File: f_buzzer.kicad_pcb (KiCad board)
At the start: 2 copper layers, 71.5 x 44 mm, 0 parts

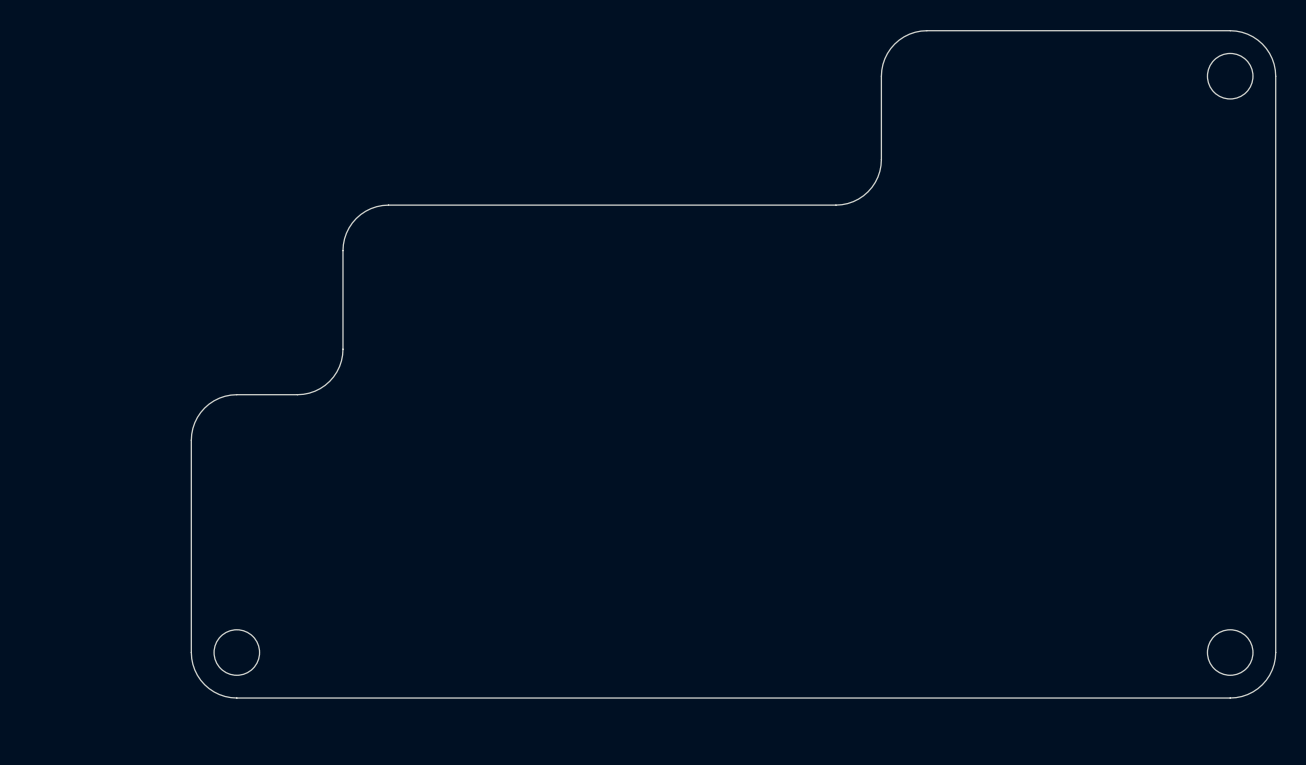
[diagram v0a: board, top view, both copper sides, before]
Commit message: Rev1
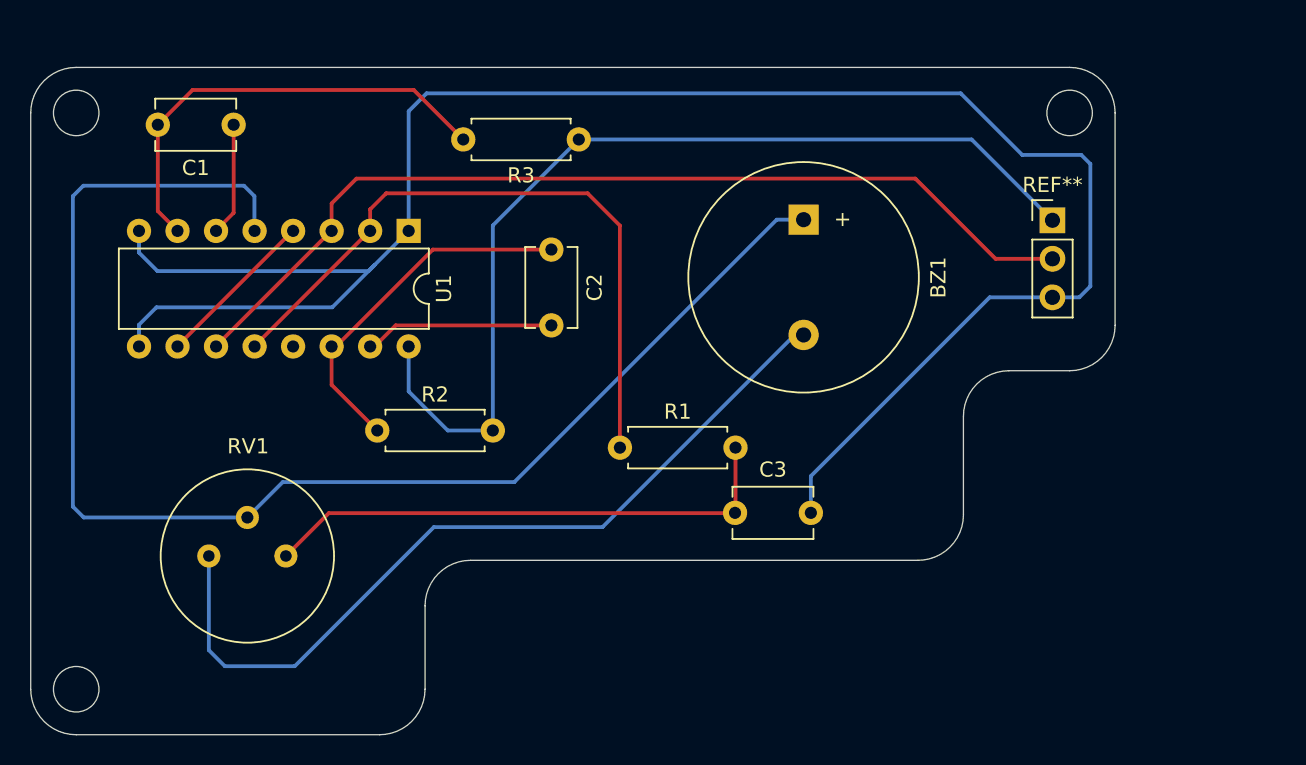
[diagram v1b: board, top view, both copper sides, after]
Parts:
- added BZ1: Buzzer, Buzzer_Beeper:Buzzer_15x7.5RM7.6, F.Cu at (165.2, 86.2)
- added C1: C, Capacitor_THT:C_Disc_D5.1mm_W3.2mm_P5.00mm, F.Cu at (127.6, 79.9)
- added C2: C, Capacitor_THT:C_Disc_D5.1mm_W3.2mm_P5.00mm, F.Cu at (148.5, 88.2)
- added C3: C, Capacitor_THT:C_Disc_D5.1mm_W3.2mm_P5.00mm, F.Cu at (160.7, 105.5)
- added R1: 330, Resistor_THT:R_Axial_DIN0207_L6.3mm_D2.5mm_P7.62mm_Horizontal, F.Cu at (153.1, 101.2)
- added R2: 27K, Resistor_THT:R_Axial_DIN0207_L6.3mm_D2.5mm_P7.62mm_Horizontal, F.Cu at (137.1, 100.1)
- added R3: 27K, Resistor_THT:R_Axial_DIN0207_L6.3mm_D2.5mm_P7.62mm_Horizontal, F.Cu at (150.3, 80.9)
- added REF**: PinHeader_1x03_P2.54mm_Horizontal, f_buzzer:PinHeader_1x03_P2.54mm_Horizontal, F.Cu at (181.6, 86.2)
- added RV1: 20K, f_buzzer:Potentiometer_Bourns_3345P_Horizontal, F.Cu at (128.5, 108.4)
- added U1: SN74123N, Package_DIP:DIP-16_W7.62mm, F.Cu at (139.1, 86.9)
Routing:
- net GND: track 0.00 -> 128.9 mm
- net Net-(BZ1-Pad1): track 0.00 -> 91.9 mm
- net VCC: track 0.00 -> 64.6 mm
- net /DVR: track 0.00 -> 63.3 mm
- net Net-(BZ1-Pad2): track 0.00 -> 54.9 mm
- net Net-(R1-Pad1): track 0.00 -> 44.9 mm
- net Net-(C3-Pad1): track 0.00 -> 34.6 mm
- net Net-(C1-Pad2): track 0.00 -> 30.0 mm
- net Net-(C2-Pad1): track 0.00 -> 24.1 mm
- net Net-(C2-Pad2): track 0.00 -> 12.7 mm
- net Net-(U1-Pad10): track 0.00 -> 11.1 mm
- net Net-(C1-Pad1): track 0.00 -> 7.46 mm
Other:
- outline, holes or cut-outs redrawn
